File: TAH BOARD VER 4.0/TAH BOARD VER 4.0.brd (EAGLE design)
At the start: 96.8 x 68 mm, 9 parts, among them M1 ARDUINO_R3_ICSP_NODIM

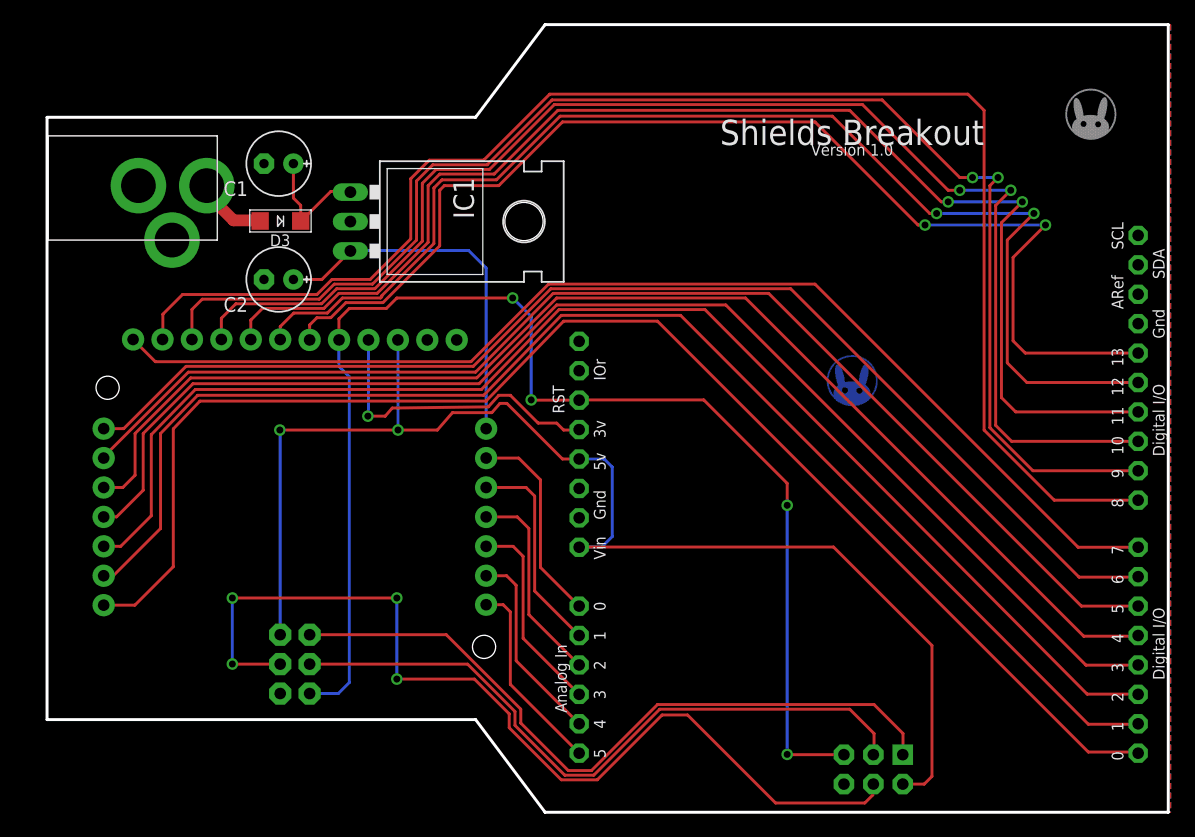
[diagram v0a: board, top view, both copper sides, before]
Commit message: TAH Shields new version update
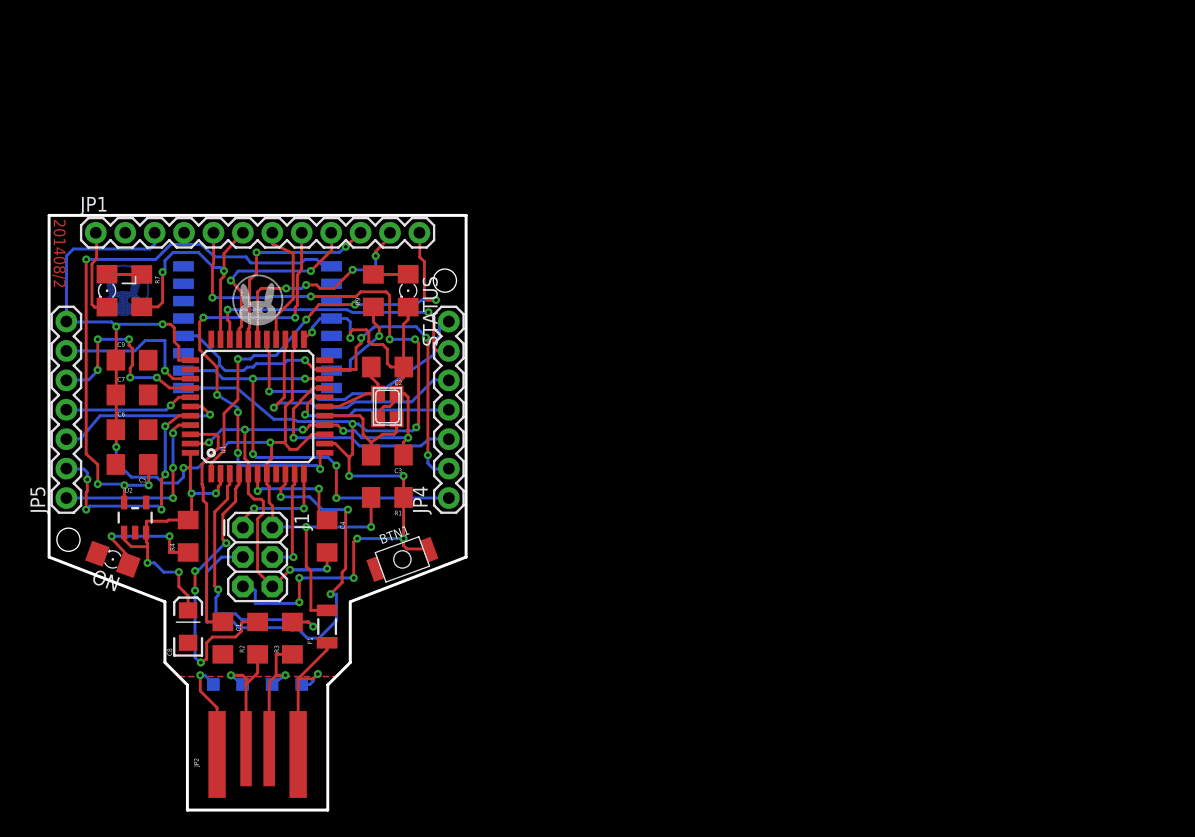
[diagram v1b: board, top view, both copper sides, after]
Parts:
- removed D3: 1N4148, 1n4148 diode sot 23:SMADIODE
- removed IC1: (no value), SparkFun-PowerIC:TO-220-ALT
- removed M1: ARDUINO_R3_ICSP_NODIM, adafruit:ARDUINOR3_ICSP_NODIM
- removed U$2: (no value), TAH:TAHLOGO
- removed U$4: (no value), TAH:TAH_LOGO_ETCHED
- added BLE: (no value), HM-11:BC05B-SMD
- added BTN1: SPST.B3U-1000P(M), omron:B3U-1000P(M)
- added C3: 18pF, SparkFun-Capacitors:1206
- added C4, C5: 1uF, SparkFun-Capacitors:1206
- added C6, C7, C9: 0.1uF, SparkFun-Capacitors:1206
- added C8: 10uF, SparkFun:EIA3216
- added F1: PTCSMD, SparkFun:PTC-1206
- added J1: AVR_SPI_PRG, SparkFun:2X3
- added JP1: M12PTH, SparkFun-Connectors:1X12
- added JP2: USBPCB, SparkFun-Connectors:USB-A-PCB
- added JP4, JP5: (no value), SparkFun-Connectors:1X07
- added L: Yellow, 1n4148 diode sot 23:1206
- added ON: Green, 1n4148 diode sot 23:1206
- added Q1: (no value), adafruit:NX3225
- added R1: 10k, SparkFun-Resistors:1206
- added R2, R3: 22, SparkFun-Resistors:1206
- added R4, R7: 1k, SparkFun-Resistors:1206
- added R9: 470, SparkFun-Resistors:1206
- added STATUS: Blue, 1n4148 diode sot 23:1206
- added TP1, TP2, TP3, TP4: TPTP11SQ, testpad:TP11SQ
- added U1: ATMEGA32U4, FTDI modifed:SPARKFUN-DIGITALIC_TQFP44
- added U2: 3.3V_REG_LDOSMD, SparkFun:SOT23-5
- C1: value 10uF -> 0.1uF; device Arduino Shield Pin Out:E2,5-6E -> SparkFun-Capacitors:1206
- C2: value 10uF -> 18pF; device Arduino Shield Pin Out:E2,5-6E -> SparkFun-Capacitors:1206
- U$1: value TAH_PIN_FOOTPRINT_VER1.0 -> (none); device TAH:TAH_PIN_FOOTPRINT_VER1.0 -> TAH:TAHLOGO
- U$3: value 2.1MMJACKTHM -> (none); device 1n4148 diode sot 23:PJ-102A -> TAH:TAH_LOGO_ETCHED
- moved C1 41.3 mm to (15.2, 15.0), turned to 270 degrees
- moved U$1 25.3 mm to (18.2, 44.3), flipped to the top
- moved C2 12.1 mm to (29.4, 38.4)
- moved U$3 9.14 mm to (6.60, 45.1), turned to 0 degrees
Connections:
- removed net D0: M1.D0, U$1.D0
- removed net D1: M1.D1, U$1.D1
- removed net N$4: D3.A, U$3.TIP
- removed net N$5: C1.+, D3.C, IC1.IN
- removed net RESET: M1.RESET, M1.RESET_ICSP, U$1.ICSP:RESET, U$1.RESET
- removed net VIN: C2.+, IC1.OUT, U$1.VIN
- new net AREF: C1.1, U1.42
- new net D+: JP2.USB_P, R2.1, TP2.TP
- new net D-: JP2.USB_M, R3.1, TP1.TP
- new net N$1: L.A, R7.1
- new net N$11: R9.2, STATUS.A
- new net N$2: C2.2, Q1.1, U1.17
- new net N$3: C3.2, Q1.3, U1.16
- new net N$6: R2.2, U1.4
- new net N$8: R3.2, U1.3
- new net N$9: ON.A, R4.1
- new net RST: BLE.1, BTN1.2, J1.5, JP1.5, R1.1, U1.13
- new net RX: BLE.4, JP4.2, U1.21
- new net RXLED: U1.8
- new net STATUSLED: BLE.15, R9.1
- new net TX: BLE.2, JP4.1, U1.20
- new net TXLED: U1.22
- new net UCAP: C4.1, U1.6
- new net VBUS: F1.1, JP2.5V, TP4.TP
- net 3.3V: now also BLE.9, C5.1, JP1.4, U2.5; no longer M1.3V, U$1.3.3V
- net 5V: now also C6.1, C7.1, C8.A, C9.1, F1.2, J1.2, JP1.3, JP5.7, R1.2, R4.2, U1.14, U1.2, U1.24, U1.34, U1.44, U1.7, U2.1, U2.3; no longer M1.5V, M1.5V_ICSP, M1.VIN, U$1.5V, U$1.ICSP:5V
- net A0: now also JP5.6, U1.36; no longer M1.A0, U$1.A0
- net A1: now also JP5.5, U1.37; no longer M1.A1, U$1.A1
- net A2: now also JP5.4, U1.38; no longer M1.A2, U$1.A2
- net A3: now also JP5.3, U1.39; no longer M1.A3, U$1.A3
- net A4: now also JP5.2, U1.40; no longer M1.A4, U$1.A4
- net A5: now also JP5.1, U1.41; no longer M1.A5, U$1.A5
- net D10: now also JP1.9, U1.30; no longer M1.D10, U$1.D10
- net D11: now also JP1.8, U1.12; no longer M1.D11, U$1.D11
- net D12: now also JP1.7, U1.26; no longer M1.D12, U$1.D12
- net D13: now also JP1.6, R7.2, U1.32; no longer M1.D13, U$1.D13
- net D2: now also JP4.3, U1.19; no longer M1.D2, U$1.D2
- net D3: now also JP4.4, U1.18; no longer M1.D3, U$1.D3
- net D4: now also JP4.5, U1.25; no longer M1.D4, U$1.D4
- net D5: now also JP4.6, U1.31; no longer M1.D5, U$1.D5
- net D6: now also JP4.7, U1.27; no longer M1.D6, U$1.D6
- net D7: now also JP1.12, U1.1; no longer M1.D7, U$1.D7
- net D8: now also JP1.11, U1.28; no longer M1.D8, U$1.D8
- net D9: now also JP1.10, U1.29; no longer M1.D9, U$1.D9
- net GND: now also BLE.12, BTN1.1, C1.2, C2.1, C3.1, C4.2, C5.2, C6.2, C7.2, C8.C, C9.2, J1.6, JP1.1, JP1.2, JP2.GND, L.C, ON.C, Q1.2, Q1.4, STATUS.C, TP3.TP, U1.15, U1.23, U1.33, U1.35, U1.43, U1.5, U2.2; no longer C1.-, C2.-, IC1.GND, M1.GND, M1.GND@1, M1.GND@2, M1.GND@3, U$1.GND1, U$1.GND2, U$1.ICSP:GND, U$3.RING, U$3.RING_SW
- net MISO: now also J1.1, U1.11; no longer M1.MISO, U$1.MISO
- net MOSI: now also J1.4, U1.10; no longer M1.MOSI, U$1.MOSI
- net SCK: now also J1.3, U1.9; no longer M1.SCK, U$1.SCK
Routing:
- net D0: track 122.0 -> 0.00 mm
- net D1: track 118.2 -> 0.00 mm
- net RESET: track 114.2 -> 0.00 mm, vias 4 -> 0
- net D8: track 128.0 -> 19.0 mm, vias 0 -> 4
- net D9: track 121.7 -> 17.5 mm
- net D10: track 117.5 -> 16.9 mm
- net RST: track 0.00 -> 97.4 mm, vias 0 -> 13
- net D3: track 112.7 -> 15.4 mm, vias 0 -> 1
- net D2: track 115.8 -> 19.9 mm, vias 0 -> 1
- net D12: track 106.0 -> 11.0 mm, vias 2 -> 0
- net GND: track 0.00 -> 90.7 mm, vias 0 -> 10
- net D4: track 110.3 -> 22.7 mm, vias 0 -> 1
- net D5: track 106.5 -> 24.7 mm, vias 0 -> 2
- net D6: track 104.6 -> 24.0 mm, vias 0 -> 1
- net D13: track 101.3 -> 21.7 mm
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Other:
- board size 96.8 x 68 mm -> 36 x 51.3 mm
- board text added: "10"
- board text added: "11"
- board text added: "12"
- board text added: "13"
- board text added: "2"
- board text added: "201408/2"
- board text added: "3"
- board text added: "3.3V"
- board text added: "4"
- board text added: "5"
- board text added: "5V"
- board text added: "6"
- board text added: "7"
- board text added: "8"
- board text added: "9"
- board text added: "A0"
- board text added: "A1"
- board text added: "A2"
- board text added: "A3"
- board text added: "A4"
- board text added: "A5"
- board text added: "GND"
- board text added: "ICSP"
- board text added: "L13"
- board text added: "ON"
- board text added: "RST"
- board text added: "RX"
- board text added: "Reset"
- board text added: "STATUS"
- board text added: "TAH"
- board text added: "TX"
- board text added: "VIN"
- board text added: "Ver. 1.0"
- board text added: "http://tah.io/start"
- board text added: "~"
- board text removed: "7-12V"
- board text removed: "7805"
- board text removed: "C1"
- board text removed: "C2"
- board text removed: "D3"
- board text removed: "POWER"
- board text removed: "Shields Breakout"
- board text removed: "Version 1.0"
- board text removed: "http://www.tah.io/start"
